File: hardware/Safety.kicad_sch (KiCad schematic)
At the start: 12 parts, among them K1 IMB03ITS, Q6 2N7002, Q8 2N7002, Q9 2N7002, U3 74AUP1G32

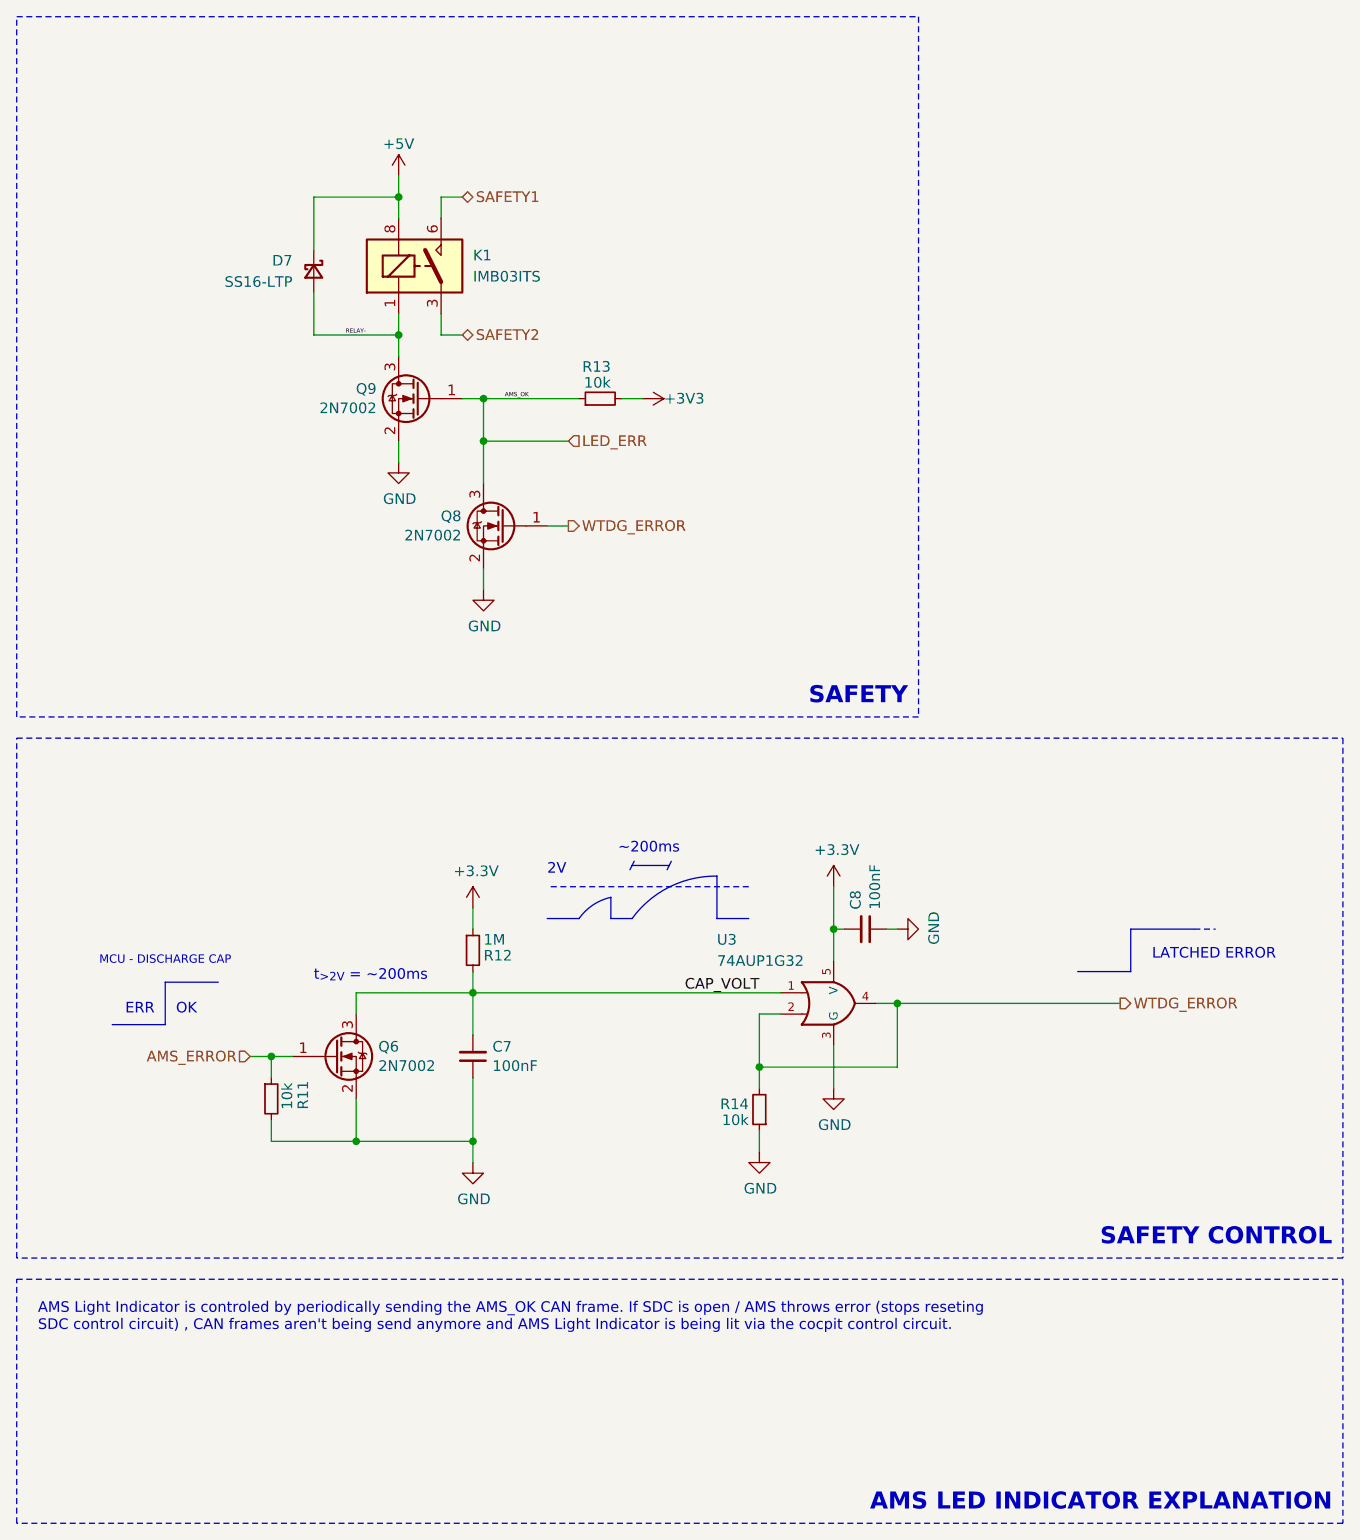
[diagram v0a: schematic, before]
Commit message: sync
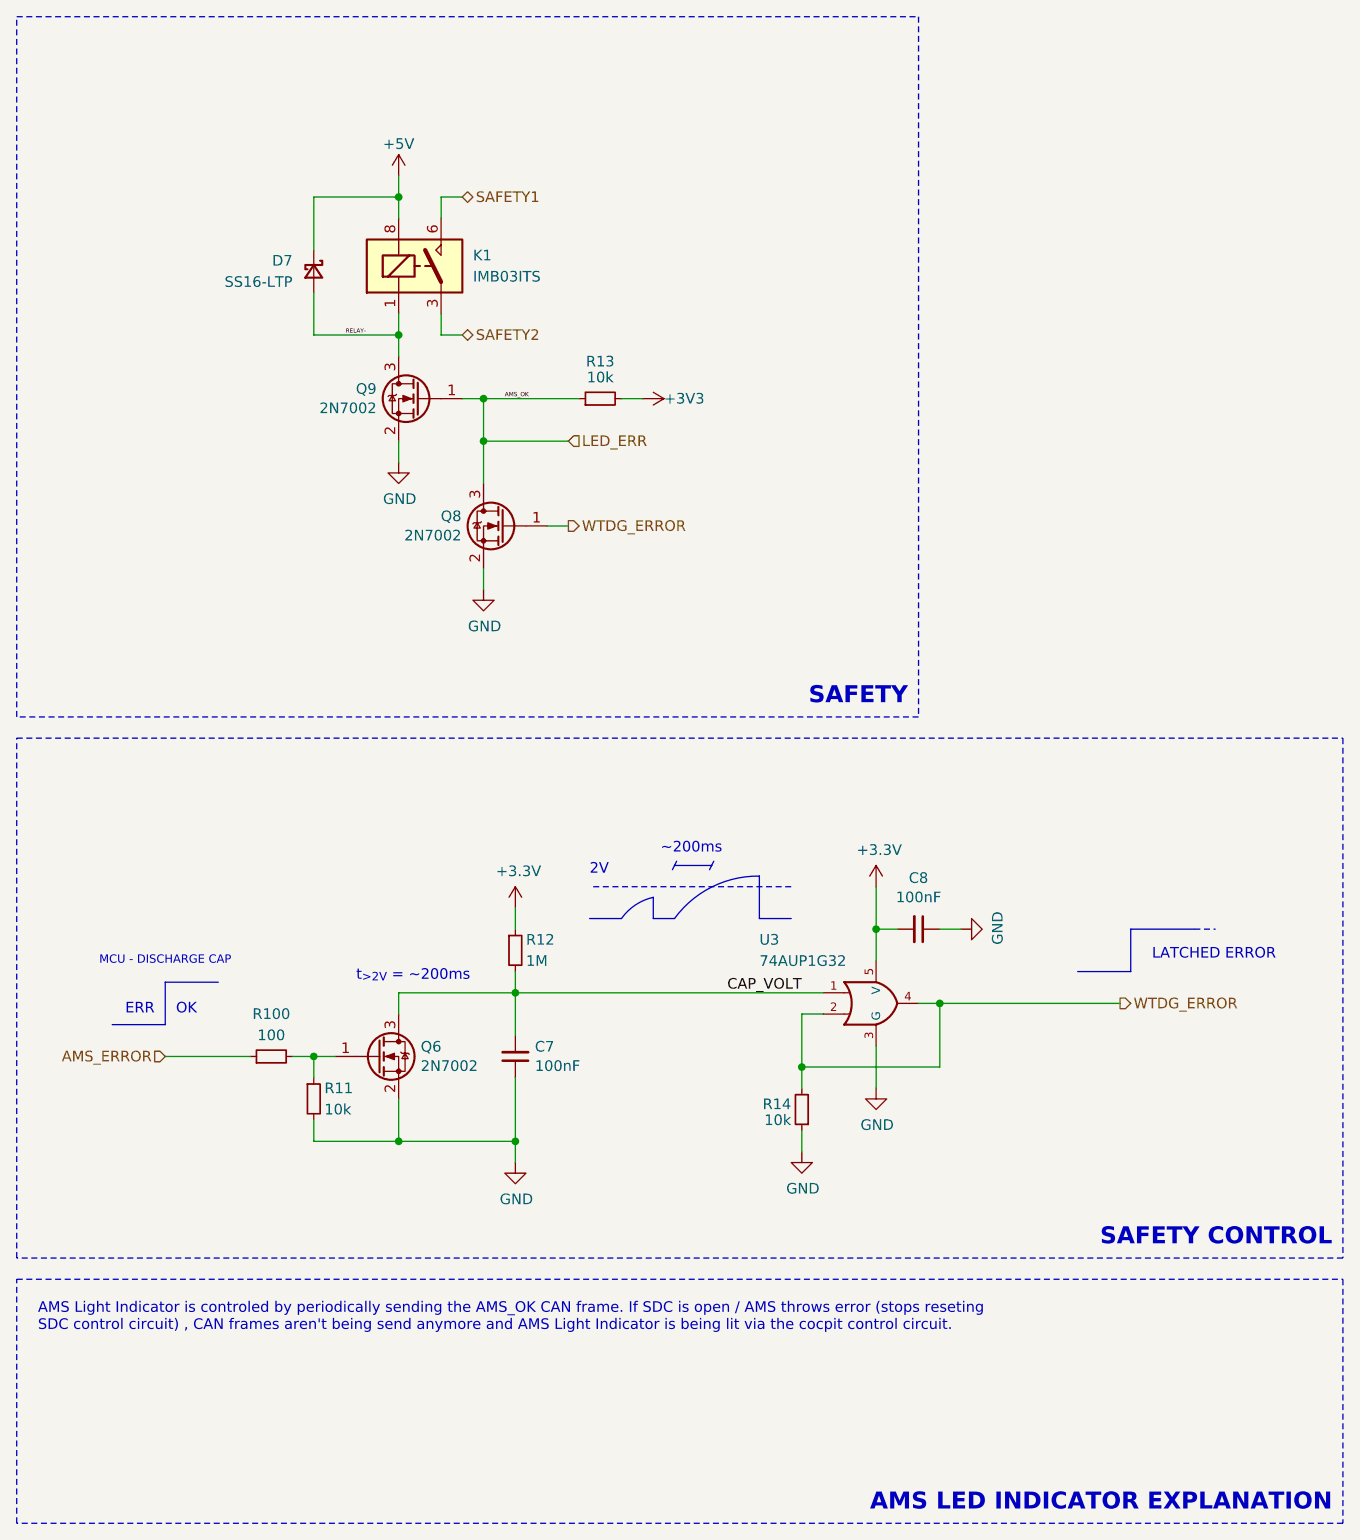
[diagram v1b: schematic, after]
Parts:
- added R100: 100, Resistor_SMD:R_0603_1608Metric, symbol Device:R_Small
- C7, C8: Mouser Price/Stock (none) -> https://www.mouser.pl/ProductDetail/KEMET/C0603C104J3RACTU?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
- R11, R13, R14: Mouser Price/Stock (none) -> https://www.mouser.pl/ProductDetail/YAGEO/RT0603DRE07100KL?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
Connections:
- net AMS_ERROR: now also R100.1; no longer Q6.1 (G), R11.1
- new net: Q6.1 (G), R100.2, R11.1
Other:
- moved on the sheet: C7, C8, Q6, R11, R12, R14, U3
